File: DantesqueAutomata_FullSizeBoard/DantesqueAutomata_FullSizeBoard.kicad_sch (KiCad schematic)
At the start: 2 parts, among them J1 Conn_02x17_Odd_Even, U1 ESP32-DevKitC

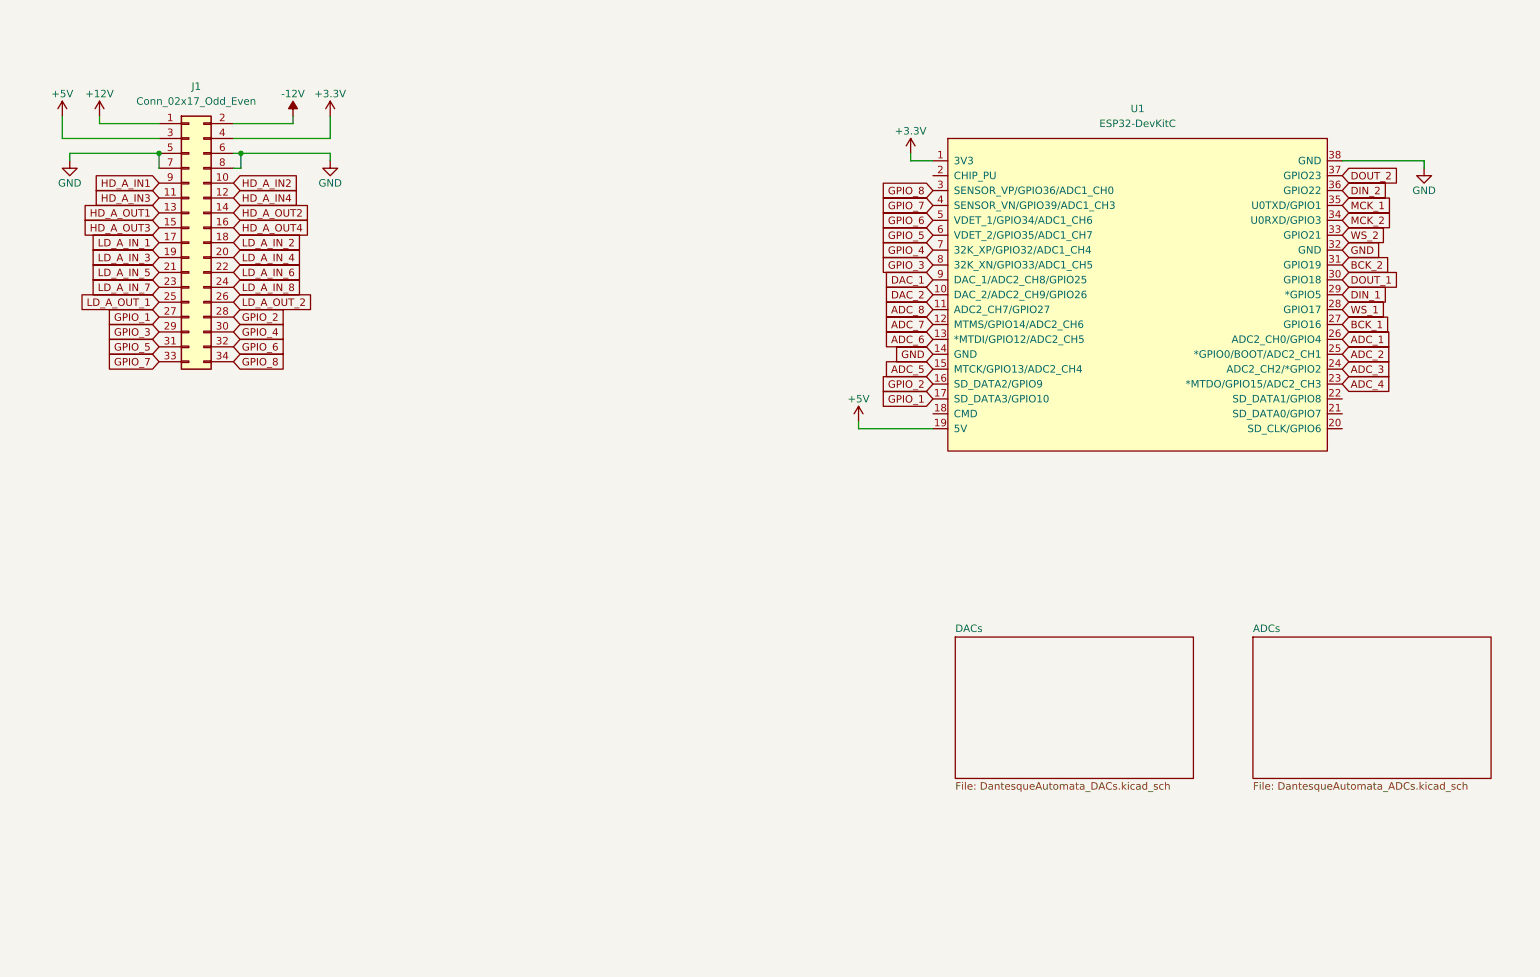
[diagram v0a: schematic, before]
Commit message: FullSizeBoard Revision 1 finished
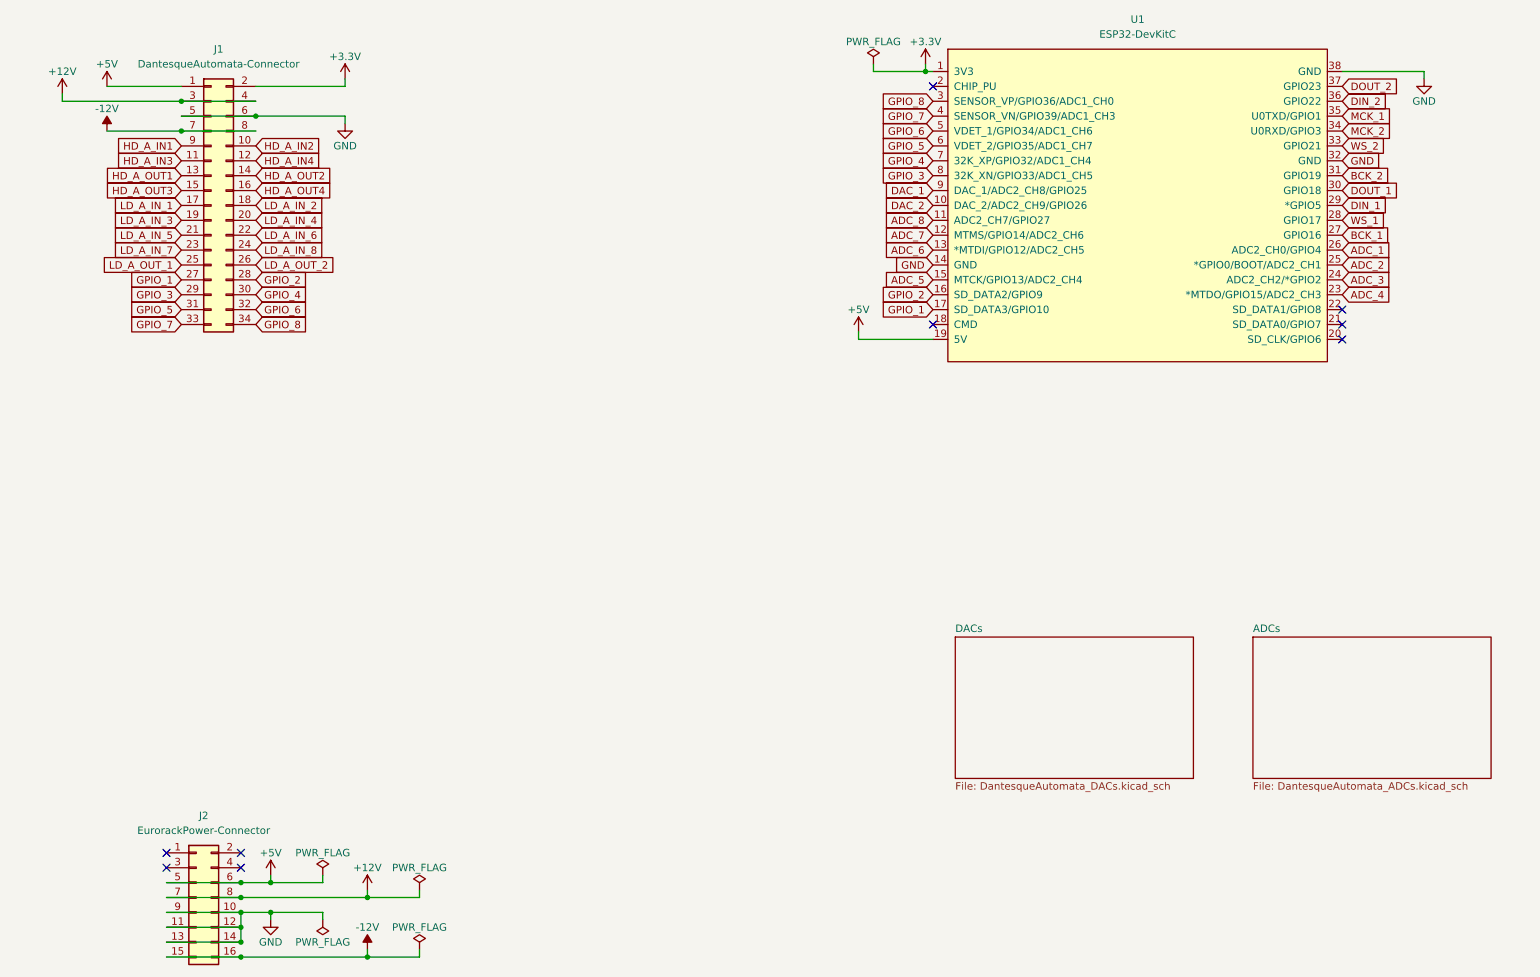
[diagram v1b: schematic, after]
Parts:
- added J2: EurorackPower-Connector, Connector_PinHeader_2.54mm:PinHeader_2x08_P2.54mm_Vertical, symbol Connector_Generic:Conn_02x08_Odd_Even
- J1: value Conn_02x17_Odd_Even -> DantesqueAutomata-Connector; footprint (none) -> Connector_PinHeader_2.54mm:PinHeader_2x17_P2.54mm_Vertical
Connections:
- net +12V: now also J1.3 (Pin_3), J1.4 (Pin_4), J2.7 (Pin_7), J2.8 (Pin_8); no longer J1.1 (Pin_1)
- net +3.3V: now also J1.2 (Pin_2); no longer J1.4 (Pin_4)
- net +5V: now also J1.1 (Pin_1), J2.5 (Pin_5), J2.6 (Pin_6); no longer J1.3 (Pin_3)
- net -12V: now also J1.7 (Pin_7), J1.8 (Pin_8), J2.15 (Pin_15), J2.16 (Pin_16); no longer J1.2 (Pin_2)
- net GND: now also J2.10 (Pin_10), J2.11 (Pin_11), J2.12 (Pin_12), J2.13 (Pin_13), J2.14 (Pin_14), J2.9 (Pin_9); no longer J1.7 (Pin_7), J1.8 (Pin_8)
- no-connect marks 0 -> 9
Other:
- moved on the sheet: J1, U1

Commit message: improved pcb design of full size board
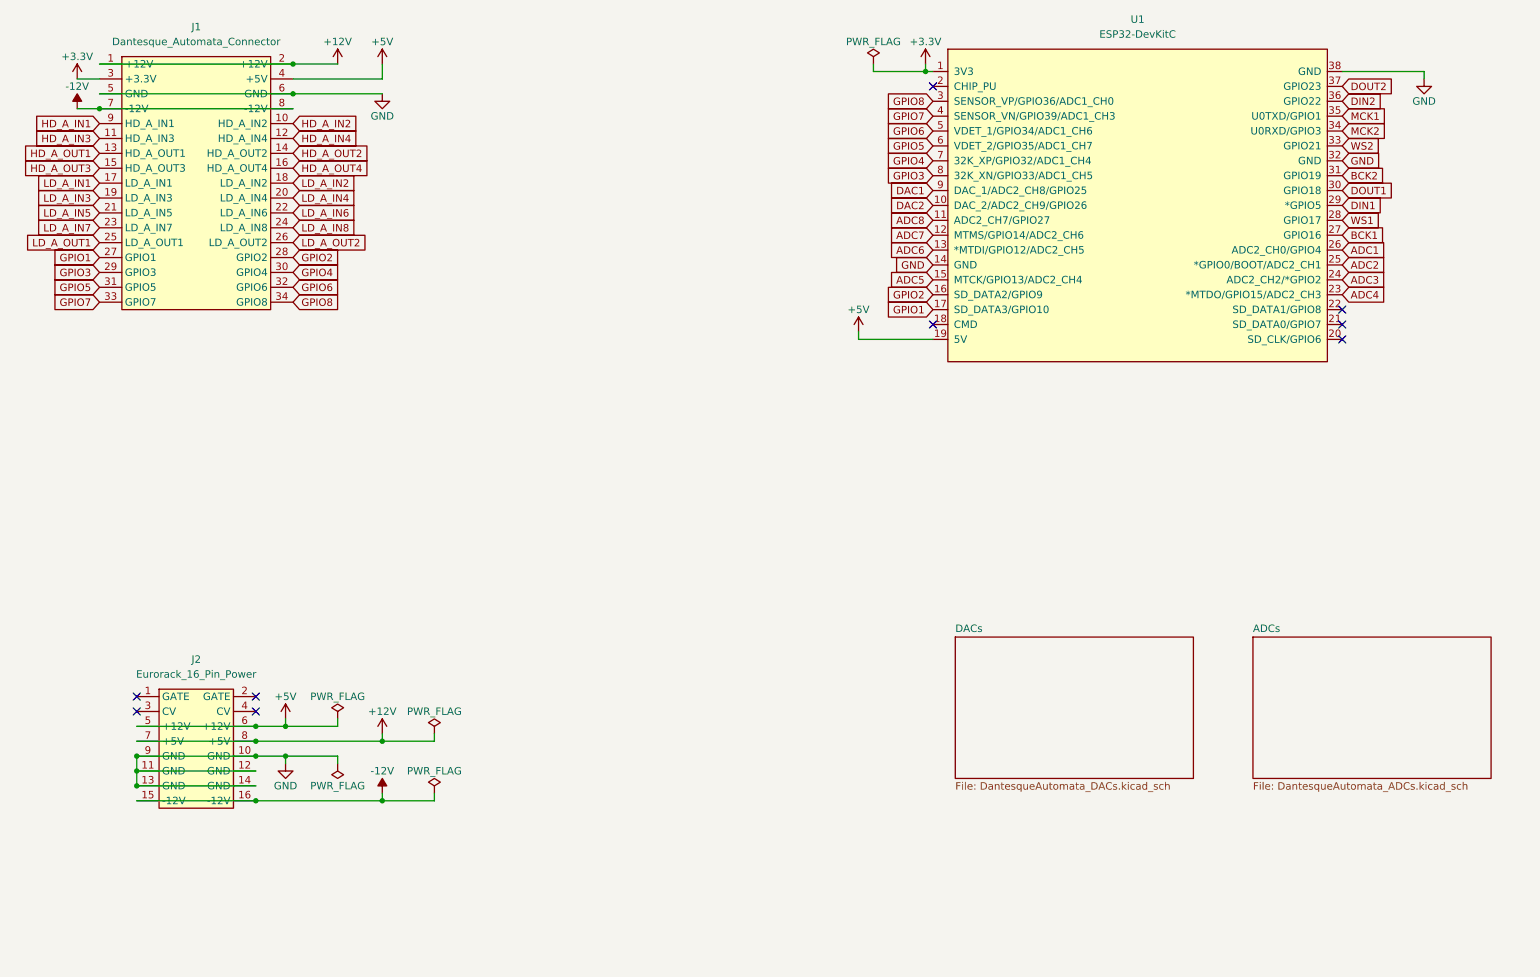
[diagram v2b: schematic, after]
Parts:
- removed J1: DantesqueAutomata-Connector, Connector_PinHeader_2.54mm:PinHeader_2x17_P2.54mm_Vertical, symbol Connector_Generic:Conn_02x17_Odd_Even
- removed J2: EurorackPower-Connector, Connector_PinHeader_2.54mm:PinHeader_2x08_P2.54mm_Vertical, symbol Connector_Generic:Conn_02x08_Odd_Even
- added J1: Dantesque_Automata_Connector, Connector_Eurorack:Dantesque_Automata_Connector, symbol Connector_Eurorack:Dantesque_Automata_Connector
- added J2: Eurorack_16_Pin_Power, Connector_Eurorack:Eurorack_16_Pin_Power, symbol Connector_Eurorack:Eurorack_16_Pin_Power
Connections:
- net +12V: now also J1.1 (+12V), J1.2 (+12V), J2.7 (+5V), J2.8 (+5V)
- net +3.3V: now also J1.3 (+3.3V)
- net +5V: now also J1.4 (+5V), J2.5 (+12V), J2.6 (+12V)
- net -12V: now also J1.7 (-12V), J1.8 (-12V), J2.15 (-12V), J2.16 (-12V)
- net GND: now also J1.5 (GND), J1.6 (GND), J2.10 (GND), J2.11 (GND), J2.12 (GND), J2.13 (GND), J2.14 (GND), J2.9 (GND)
- net HD_A_IN1: now also J1.9 (HD_A_IN1)
- net HD_A_IN2: now also J1.10 (HD_A_IN2)
- net HD_A_IN3: now also J1.11 (HD_A_IN3)
- net HD_A_IN4: now also J1.12 (HD_A_IN4)
- net HD_A_OUT1: now also J1.13 (HD_A_OUT1)
- net HD_A_OUT2: now also J1.14 (HD_A_OUT2)
- net HD_A_OUT3: now also J1.15 (HD_A_OUT3)
- net HD_A_OUT4: now also J1.16 (HD_A_OUT4)
- net ADC_1 renamed ADC1
- net ADC_2 renamed ADC2
- net ADC_3 renamed ADC3
- net ADC_4 renamed ADC4
- net ADC_5 renamed ADC5
- net ADC_6 renamed ADC6
- net ADC_7 renamed ADC7
- net ADC_8 renamed ADC8
- net BCK_1 renamed BCK1
- net BCK_2 renamed BCK2
- net DAC_1 renamed DAC1
- net DAC_2 renamed DAC2
- net DIN_1 renamed DIN1
- net DIN_2 renamed DIN2
- net DOUT_1 renamed DOUT1
- net DOUT_2 renamed DOUT2
- net GPIO_1 renamed GPIO1
- net GPIO1: now also J1.27 (GPIO1)
- net GPIO_2 renamed GPIO2
- net GPIO2: now also J1.28 (GPIO2)
- net GPIO_3 renamed GPIO3
- net GPIO3: now also J1.29 (GPIO3)
- net GPIO_4 renamed GPIO4
- net GPIO4: now also J1.30 (GPIO4)
- net GPIO_5 renamed GPIO5
- net GPIO5: now also J1.31 (GPIO5)
- net GPIO_6 renamed GPIO6
- net GPIO6: now also J1.32 (GPIO6)
- net GPIO_7 renamed GPIO7
- net GPIO7: now also J1.33 (GPIO7)
- net GPIO_8 renamed GPIO8
- net GPIO8: now also J1.34 (GPIO8)
- net MCK_1 renamed MCK1
- net MCK_2 renamed MCK2
- net WS_1 renamed WS1
- net WS_2 renamed WS2
- new net LD_A_IN1: J1.17 (LD_A_IN1)
- new net LD_A_IN2: J1.18 (LD_A_IN2)
- new net LD_A_IN3: J1.19 (LD_A_IN3)
- new net LD_A_IN4: J1.20 (LD_A_IN4)
- new net LD_A_IN5: J1.21 (LD_A_IN5)
- new net LD_A_IN6: J1.22 (LD_A_IN6)
- new net LD_A_IN7: J1.23 (LD_A_IN7)
- new net LD_A_IN8: J1.24 (LD_A_IN8)
- new net LD_A_OUT1: J1.25 (LD_A_OUT1)
- new net LD_A_OUT2: J1.26 (LD_A_OUT2)
